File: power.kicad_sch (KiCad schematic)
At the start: 28 parts, among them U1 TPS54325PWP, U2 TPS54294PWP

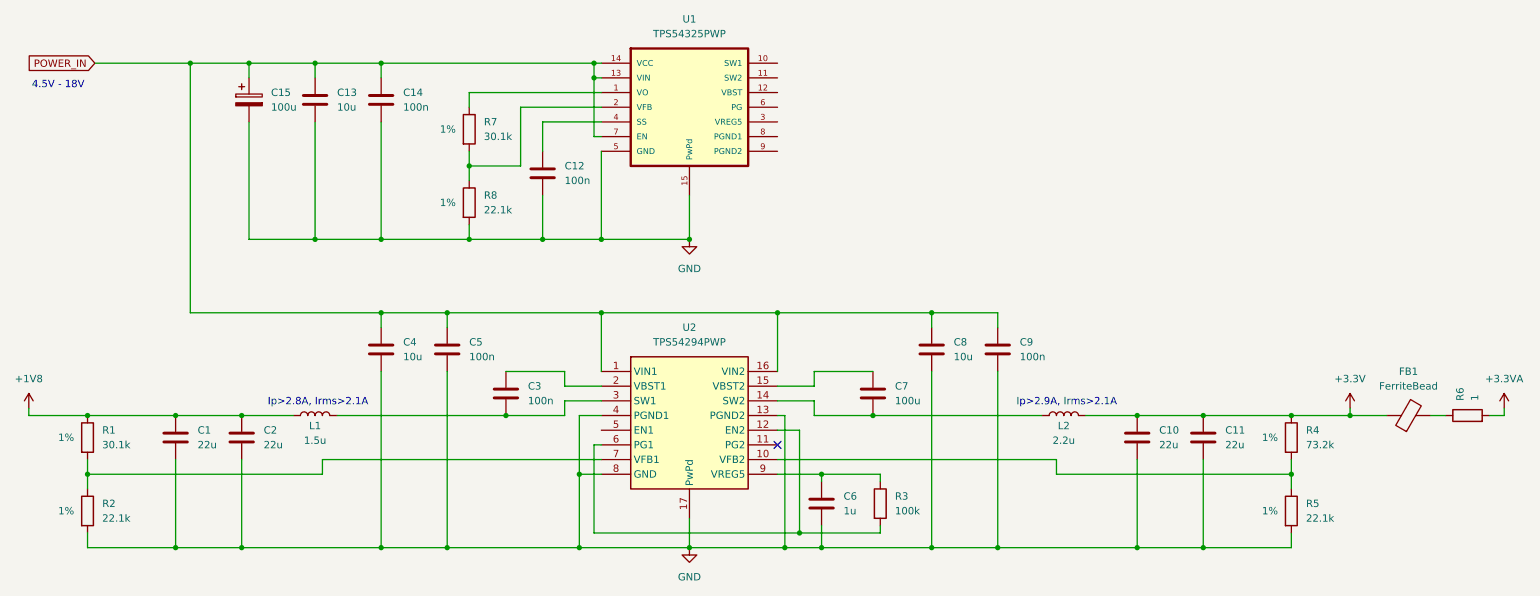
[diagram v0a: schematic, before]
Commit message: Finish power supply?
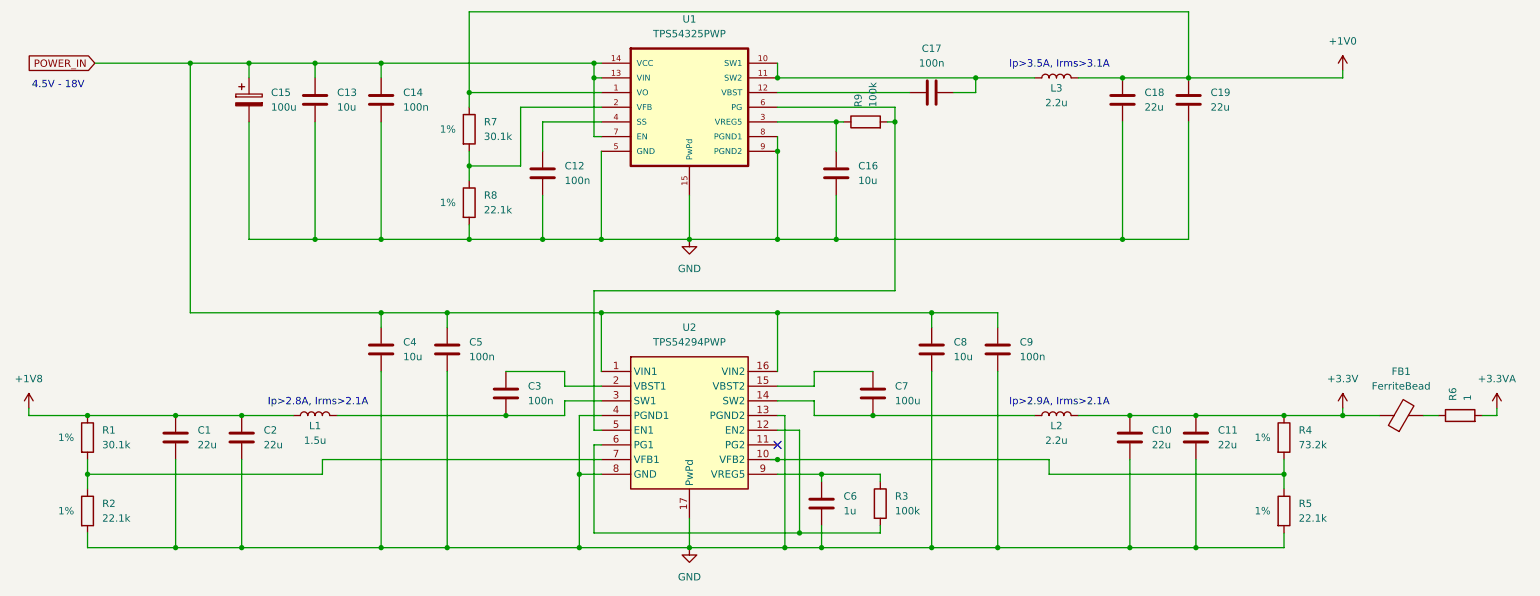
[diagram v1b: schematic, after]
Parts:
- added C16: 10u, symbol Device:C
- added C17: 100n, symbol Device:C
- added C18, C19: 22u, symbol Device:C
- added L3: 2.2u, symbol Device:L
- added R9: 100k, symbol Device:R
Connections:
- net GND: now also U1.8 (PGND1), U1.9 (PGND2), C16.2, C18.2, C19.2
- net +1V0: now reaches R7.1, U1.1 (VO)
- net +1V0: now also C18.1, C19.1, L3.2
- net at U1.10 (SW1): now also U1.11 (SW2), C17.2, L3.1
- net at U1.12 (VBST): now also C17.1
- net at U1.3 (VREG5): now also C16.1, R9.1
- net at U1.6 (PG): now also U2.5 (EN1), R9.2
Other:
- note added: "Ip>3.5A, Irms>3.1A"
- moved on the sheet: C10, C11, FB1, L2, R4, R5, R6
